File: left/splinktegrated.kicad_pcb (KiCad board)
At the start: 4 copper layers, 72.6 x 88.4 mm, 83 parts, among them J1 USB_C_Receptacle_USB2.0, J10 NA_Ribbon, J13 Conn_01x01_Socket, J14 Cirque, J15 Conn_01x01_Socket, J16 Conn_01x01_Socket, J17 Conn_01x01_Socket, J18 USB_C_Receptacle_USB2.0, J19 Conn_01x01_Socket, J20 Conn_01x01_Socket, J5 Conn_01x02, J6 Cirque, J7 NA_trackball, J8 NA_Ribbon, J9 NA_RGB, Q4 AO3401A, Q5 AO3401A, SW2 NA_SW_SPST, U1 RP2040, U2 USBLC6-2P6, U3 XC6210B332MR-G, U4 USBLC6-2P6, U5 W25Q128JVS, U6 74LVC1T45, Y1 Crystal_GND24

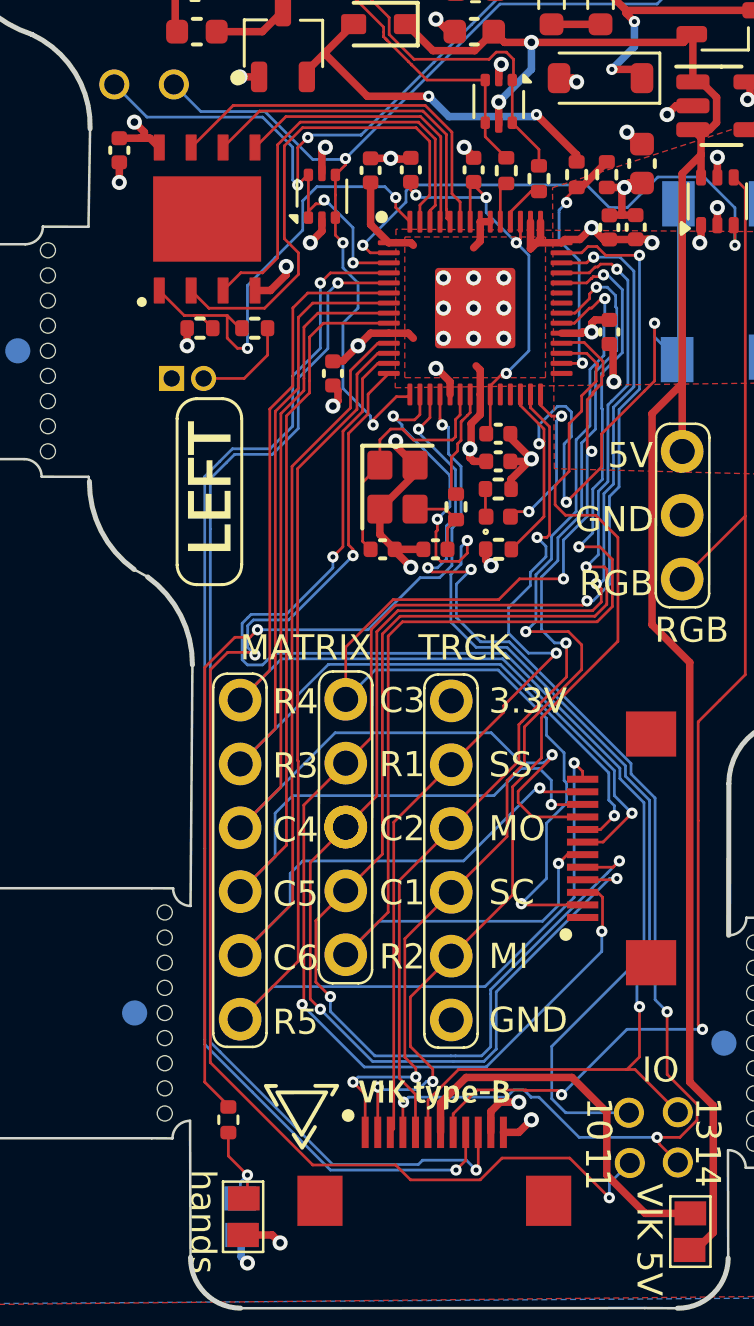
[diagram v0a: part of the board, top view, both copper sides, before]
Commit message: routing
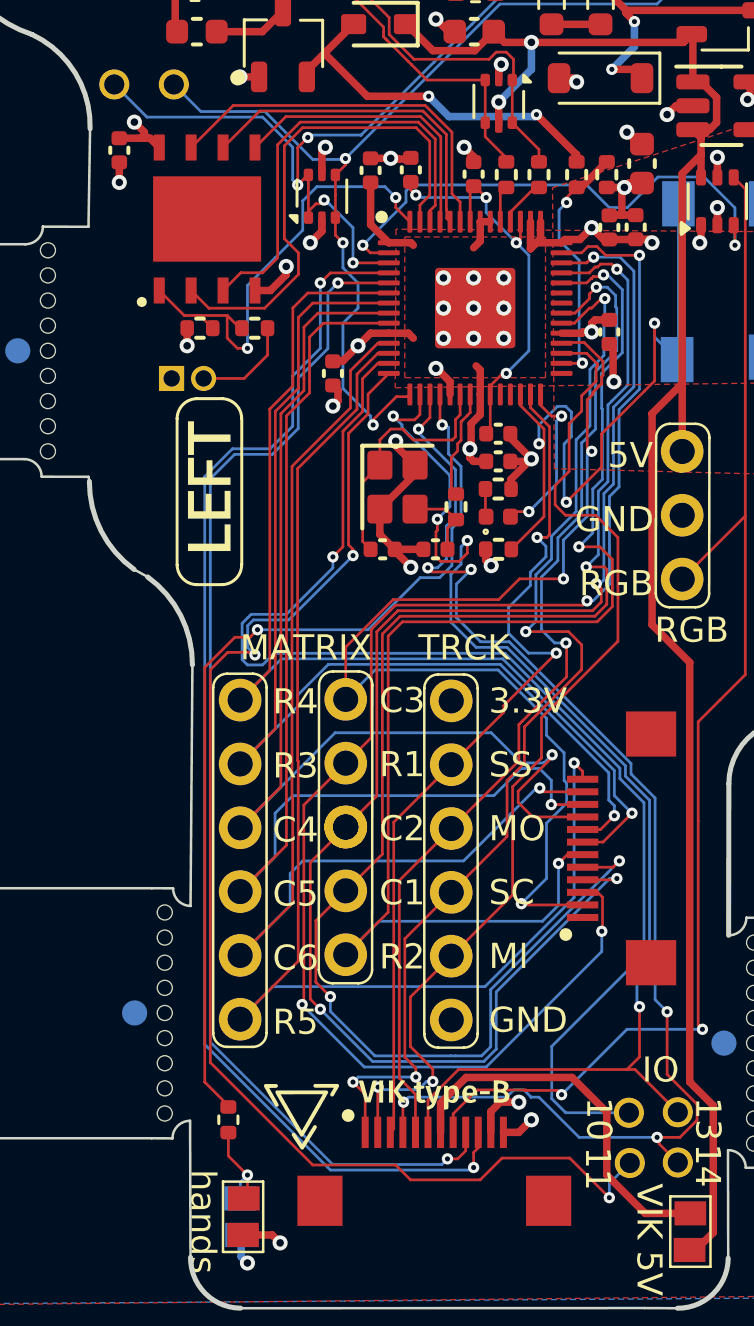
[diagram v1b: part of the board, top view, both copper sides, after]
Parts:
- moved C6 0.17 mm to (156.5, 92.7)
- moved R6 0.16 mm to (157.8, 92.7)
- moved R7 0.16 mm to (159.1, 92.7)
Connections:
- J6 pad 10: SCL -> SDA
- J6 pad 9: SDA -> SCL
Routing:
- net SCL: track 49.6 -> 48.4 mm
- net SDA: track 49.7 -> 50.3 mm
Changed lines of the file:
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@@
 	(footprint "Resistor_SMD:R_0402_1005Metric"
 		(layer "F.Cu")
-		(at 157.8 92.53 -90)
+		(at 157.8 92.69 -90)
 		(descr "Resistor SMD 0402 (1005 Metric), square (rectangular) end terminal, IPC_7351 nominal, (Body size source: IPC-SM-782 page 72, https://www.pcb-3d.com/wordpress/wp-content/uploads/ipc-sm-782a_amendment_1_and_2.pdf), generated with kicad-footprint-generator")
 		(tags "resistor")
@@
 	(footprint "Resistor_SMD:R_0402_1005Metric"
 		(layer "F.Cu")
-		(at 159.1 92.85 -90)
+		(at 159.1 92.69 -90)
 		(descr "Resistor SMD 0402 (1005 Metric), square (rectangular) end terminal, IPC_7351 nominal, (Body size source: IPC-SM-782 page 72, https://www.pcb-3d.com/wordpress/wp-content/uploads/ipc-sm-782a_amendment_1_and_2.pdf), generated with kicad-footprint-generator")
 		(tags "resistor")
@@
 	(footprint "Capacitor_SMD:C_0402_1005Metric"
 		(layer "F.Cu")
-		(at 156.5 92.5 90)
+		(at 156.5 92.67 90)
 		(descr "Capacitor SMD 0402 (1005 Metric), square (rectangular) end terminal, IPC_7351 nominal, (Body size source: IPC-SM-782 page 76, https://www.pcb-3d.com/wordpress/wp-content/uploads/ipc-sm-782a_amendment_1_and_2.pdf), generated with kicad-footprint-generator")
 		(tags "capacitor")
@@
 			(size 0.28 1.25)
 			(layers "F.Cu" "F.Mask" "F.Paste")
-			(net 53 "SDA")
+			(net 54 "SCL")
 			(pinfunction "Pin_9")
 			(pintype "passive")
@@
 			(size 0.28 1.25)
 			(layers "F.Cu" "F.Mask" "F.Paste")
-			(net 54 "SCL")
+			(net 53 "SDA")
 			(pinfunction "Pin_10")
 			(pintype "passive")
@@
 			)
 		)
+		(property ki_fp_filters "MountingHole*Pad*")
+		(sheetname "/")
+		(sheetfile "splinktegrated.kicad_sch")
 		(attr exclude_from_pos_files dnp)
 		(fp_circle
@@
 			)
 		)
+		(property ki_fp_filters "Connector*:*_1x??_*")
+		(sheetname "/")
+		(sheetfile "splinktegrated.kicad_sch")
 		(attr through_hole exclude_from_pos_files exclude_from_bom dnp)
 		(fp_line
@@
 			)
 		)
+		(property ki_fp_filters "Connector*:*_1x??_*")
+		(sheetname "/")
+		(sheetfile "splinktegrated.kicad_sch")
 		(attr through_hole exclude_from_pos_files exclude_from_bom dnp)
 		(fp_line
@@
 			)
 		)
+		(property ki_fp_filters "MountingHole*Pad*")
+		(sheetname "/")
+		(sheetfile "splinktegrated.kicad_sch")
 		(attr exclude_from_pos_files dnp)
 		(fp_circle
@@
 			)
 		)
+		(property ki_fp_filters "Connector*:*_1x??_*")
+		(sheetname "/")
+		(sheetfile "splinktegrated.kicad_sch")
 		(attr through_hole exclude_from_pos_files exclude_from_bom dnp)
 		(fp_line
@@
 			)
 		)
+		(property ki_fp_filters "Connector*:*_1x??_*")
+		(sheetname "/")
+		(sheetfile "splinktegrated.kicad_sch")
 		(attr through_hole exclude_from_pos_files exclude_from_bom dnp)
 		(fp_line
@@
 	)
 	(segment
-		(start 156.185 131.915)
-		(end 156.185 130.8)
+		(start 156.685 131.415)
+		(end 156.685 130.8)
 		(width 0.11)
 		(layer "F.Cu")
@@
 	)
 	(segment
-		(start 150.8 96.6)
-		(end 150.4 97)
+		(start 156.5 131.6)
+		(end 156.685 131.415)
+		(width 0.11)
+		(layer "F.Cu")
+		(net 53)
+	)
+	(segment
+		(start 156.5 132.2)
+		(end 156.5 131.6)
 		(width 0.11)
 		(layer "F.Cu")
@@
 	)
 	(segment
-		(start 155.8 132.3)
-		(end 156.185 131.915)
+		(start 150.8 96.6)
+		(end 150.4 97)
 		(width 0.11)
 		(layer "F.Cu")
@@
 	)
 	(via
-		(at 155.8 132.3)
+		(at 156.5 132.2)
 		(size 0.45)
 		(drill 0.2)
@@
 	)
 	(segment
-		(start 145.8 127.3)
-		(end 147.7 129.2)
-		(width 0.11)
-		(layer "B.Cu")
-		(net 53)
-	)
-	(segment
-		(start 147.7 129.2)
-		(end 150.8 132.3)
+		(start 150.4 99.6)
+		(end 150.4 97)
 		(width 0.11)
 		(layer "B.Cu")
@@
 	)
 	(segment
-		(start 146.900001 103.6)
-		(end 148.4 103.6)
+		(start 149.3 100.7)
+		(end 150.4 99.6)
 		(width 0.11)
 		(layer "B.Cu")
@@
 	)
 	(segment
-		(start 145.8 104.7)
-		(end 145.8 119.5)
+		(start 145.8 127.3)
+		(end 145.8 104.7)
 		(width 0.11)
 		(layer "B.Cu")
@@
 	)
 	(segment
-		(start 150.4 99.6)
-		(end 150.4 97)
+		(start 150.8 132.3)
+		(end 145.8 127.3)
 		(width 0.11)
 		(layer "B.Cu")
@@
 	)
 	(segment
-		(start 145.8 119.5)
-		(end 145.8 127.1)
+		(start 156.4 132.3)
+		(end 150.8 132.3)
 		(width 0.11)
 		(layer "B.Cu")
@@
 	)
 	(segment
-		(start 149.3 100.7)
-		(end 150.4 99.6)
+		(start 145.8 104.7)
+		(end 146.900001 103.6)
 		(width 0.11)
 		(layer "B.Cu")
@@
 	)
 	(segment
-		(start 150.8 132.3)
-		(end 155.8 132.3)
+		(start 146.900001 103.6)
+		(end 148.4 103.6)
 		(width 0.11)
 		(layer "B.Cu")
@@
 	)
 	(segment
-		(start 146.4 104.1)
-		(end 146.900001 103.6)
+		(start 156.5 132.2)
+		(end 156.4 132.3)
 		(width 0.11)
 		(layer "B.Cu")
@@
 	)
 	(segment
-		(start 145.8 127.1)
-		(end 145.8 127.3)
+		(start 155.864293 131.855707)
+		(end 156.185 131.535)
 		(width 0.11)
-		(layer "B.Cu")
-		(net 53)
+		(layer "F.Cu")
+		(net 54)
 	)
 	(segment
-		(start 146.4 104.1)
-		(end 145.8 104.7)
-		(width 0.11)
-		(layer "B.Cu")
-		(net 53)
-	)
-	(segment
-		(start 156.685 132.215)
-		(end 156.685 130.8)
+		(start 155.459109 131.855707)
+		(end 155.864293 131.855707)
 		(width 0.11)
 		(layer "F.Cu")
@@
 	)
 	(segment
-		(start 156.6 132.3)
-		(end 156.685 132.215)
+		(start 156.185 131.535)
+		(end 156.185 130.8)
 		(width 0.11)
 		(layer "F.Cu")
@@
 	)
 	(via
-		(at 156.6 132.3)
+		(at 155.459109 131.855707)
 		(size 0.45)
 		(drill 0.2)
@@
 	)
 	(segment
-		(start 156.209 131.909)
-		(end 156.6 132.3)
-		(width 0.11)
-		(layer "B.Cu")
-		(net 54)
-	)
-	(segment
-		(start 146.991542 103.821)
-		(end 148.491541 103.821)
-		(width 0.11)
-		(layer "B.Cu")
-		(net 54)
-	)
-	(segment
-		(start 154.47 131.909)
-		(end 156.209 131.909)
-		(width 0.11)
-		(layer "B.Cu")
-		(net 54)
-	)
-	(segment
-		(start 150.7 99.612542)
-		(end 150.7 97.4)
-		(width 0.11)
-		(layer "B.Cu")
-		(net 54)
-	)
-	(segment
-		(start 148.491541 103.821)
-		(end 149.521 102.791542)
-		(width 0.11)
-		(layer "B.Cu")
-		(net 54)
-	)
-	(segment
-		(start 146.656271 104.156271)
-		(end 146.021 104.791542)
+		(start 150.891542 132.079)
+		(end 146.021 127.208458)
 		(width 0.11)
 		(layer "B.Cu")
@@
 	)
 	(segment
-		(start 146.021 127.2)
-		(end 146.021 127.208458)
+		(start 149.521 102.791542)
+		(end 149.521 100.791542)
 		(width 0.11)
 		(layer "B.Cu")
@@
 	)
 	(segment
-		(start 146.656271 104.156271)
+		(start 146.021 104.791542)
 		(end 146.991542 103.821)
 		(width 0.11)
@@
 	)
 	(segment
-		(start 154.3 132.079)
-		(end 154.47 131.909)
+		(start 155.235816 132.079)
+		(end 150.891542 132.079)
 		(width 0.11)
 		(layer "B.Cu")
@@
 	)
 	(segment
-		(start 149.521 102.791542)
-		(end 149.521 100.791542)
+		(start 155.459109 131.855707)
+		(end 155.235816 132.079)
 		(width 0.11)
 		(layer "B.Cu")
@@
 	)
 	(segment
-		(start 146.021 106.8)
-		(end 146.021 113.9)
+		(start 148.491541 103.821)
+		(end 149.521 102.791542)
 		(width 0.11)
 		(layer "B.Cu")
@@
 	)
 	(segment
-		(start 146.021 127.208458)
-		(end 146.406271 127.593729)
-		(width 0.11)
-		(layer "B.Cu")
-		(net 54)
-	)
-	(segment
-		(start 146.021 113.9)
-		(end 146.021 118.2)
-		(width 0.11)
-		(layer "B.Cu")
-		(net 54)
-	)
-	(segment
 		(start 150.7 97.4)
 		(end 151.1 97)
@@
 	)
 	(segment
-		(start 150.891542 132.079)
-		(end 154.3 132.079)
-		(width 0.11)
-		(layer "B.Cu")
-		(net 54)
-	)
-	(segment
-		(start 146.406271 127.593729)
-		(end 150.891542 132.079)
+		(start 146.991542 103.821)
+		(end 148.491541 103.821)
 		(width 0.11)
 		(layer "B.Cu")
@@
 	)
 	(segment
-		(start 146.021 104.791542)
-		(end 146.021 106.8)
+		(start 150.7 99.612542)
+		(end 150.7 97.4)
 		(width 0.11)
 		(layer "B.Cu")
@@
 	)
 	(segment
-		(start 146.021 118.2)
-		(end 146.021 127.2)
+		(start 146.021 127.208458)
+		(end 146.021 104.791542)
 		(width 0.11)
 		(layer "B.Cu")
